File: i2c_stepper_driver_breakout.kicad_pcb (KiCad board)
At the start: 2 copper layers, 23 x 28 mm, 23 parts, among them J1 Conn_01x10, J2 Conn_01x10, J3 S4B-PH-SM4-TB, U1 PCA9629A, U2 A3909, U3 MAX17291

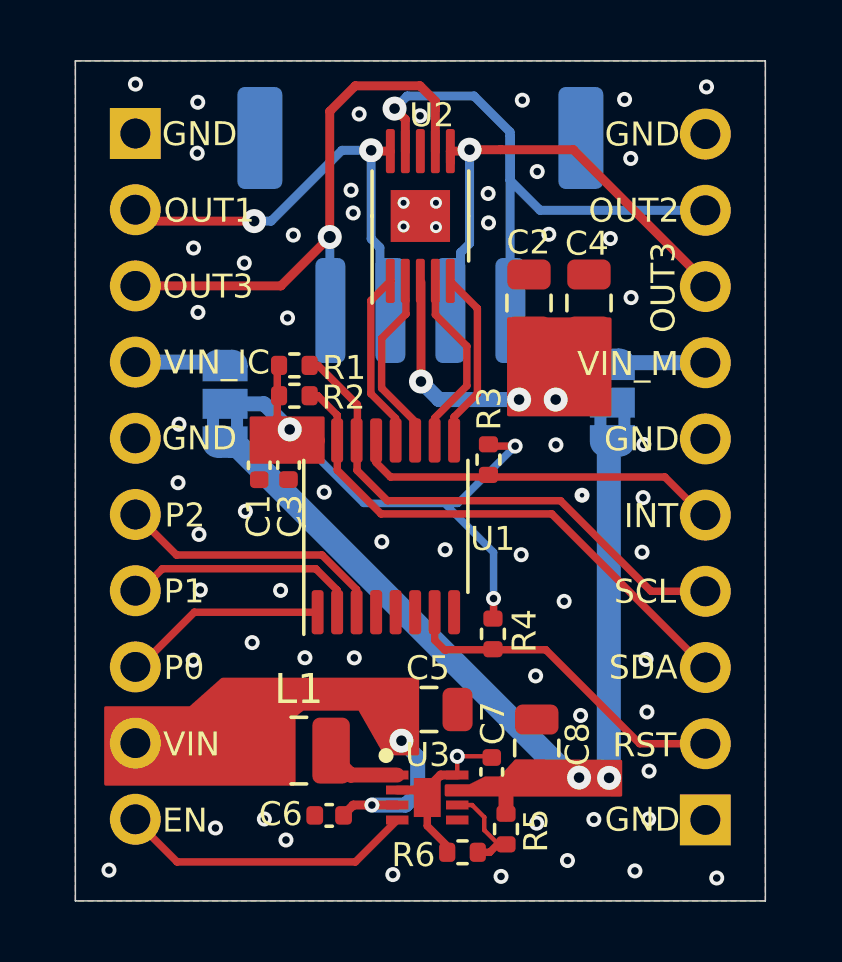
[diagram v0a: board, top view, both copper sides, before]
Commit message: Bugfixes
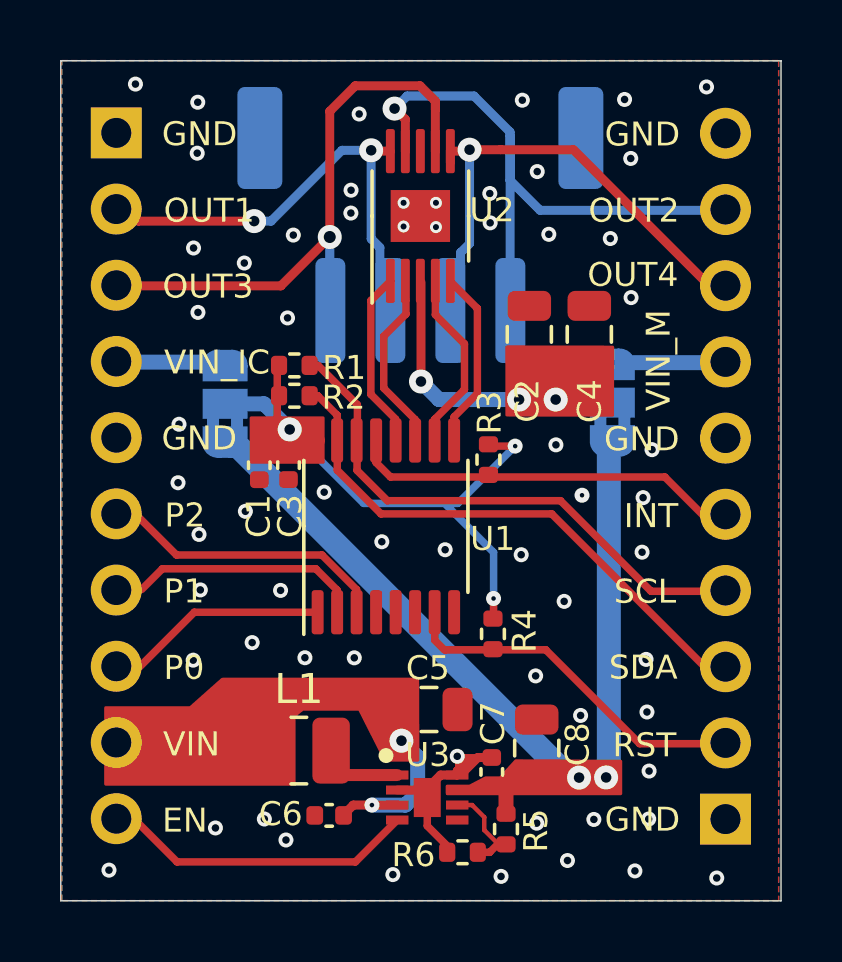
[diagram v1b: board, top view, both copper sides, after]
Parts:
- moved C2 1.05 mm to (150.1, 92.1)
- moved C4 1.05 mm to (152.1, 92.1)
- moved J2 0.67 mm to (156.7, 108.3)
- moved J1 0.64 mm to (136.4, 85.4)
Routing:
- net GND: track 6.97 -> 8.73 mm, vias 64 -> 59
- net /VIN_BOOST: track 15.6 -> 16.7 mm
- net /VBB: track 14.7 -> 13.8 mm
- net (no net): vias 0 -> 4
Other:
- board size 23 x 28 mm -> 24 x 28 mm
- net class Default: clearance 0.1 -> 0.15
- rule trace_clearance: 0.1 -> 0.15
- board text added: "OUT4"
